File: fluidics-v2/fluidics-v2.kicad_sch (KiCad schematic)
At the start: 25 parts, among them J1 PJ-063AH, J10 87832-1010, J11 87832-1010, J12 87832-1010, J13 0533980671, J14 0533980671, J15 A-DS_15_A_KG-T4S, J2 0705430001, J3 0705430001, J4 0705430001, J5 0705430001, J6 0705430001, J7 1860280, J8 87832-1010, J9 87832-1010, U2 Teensy4.1

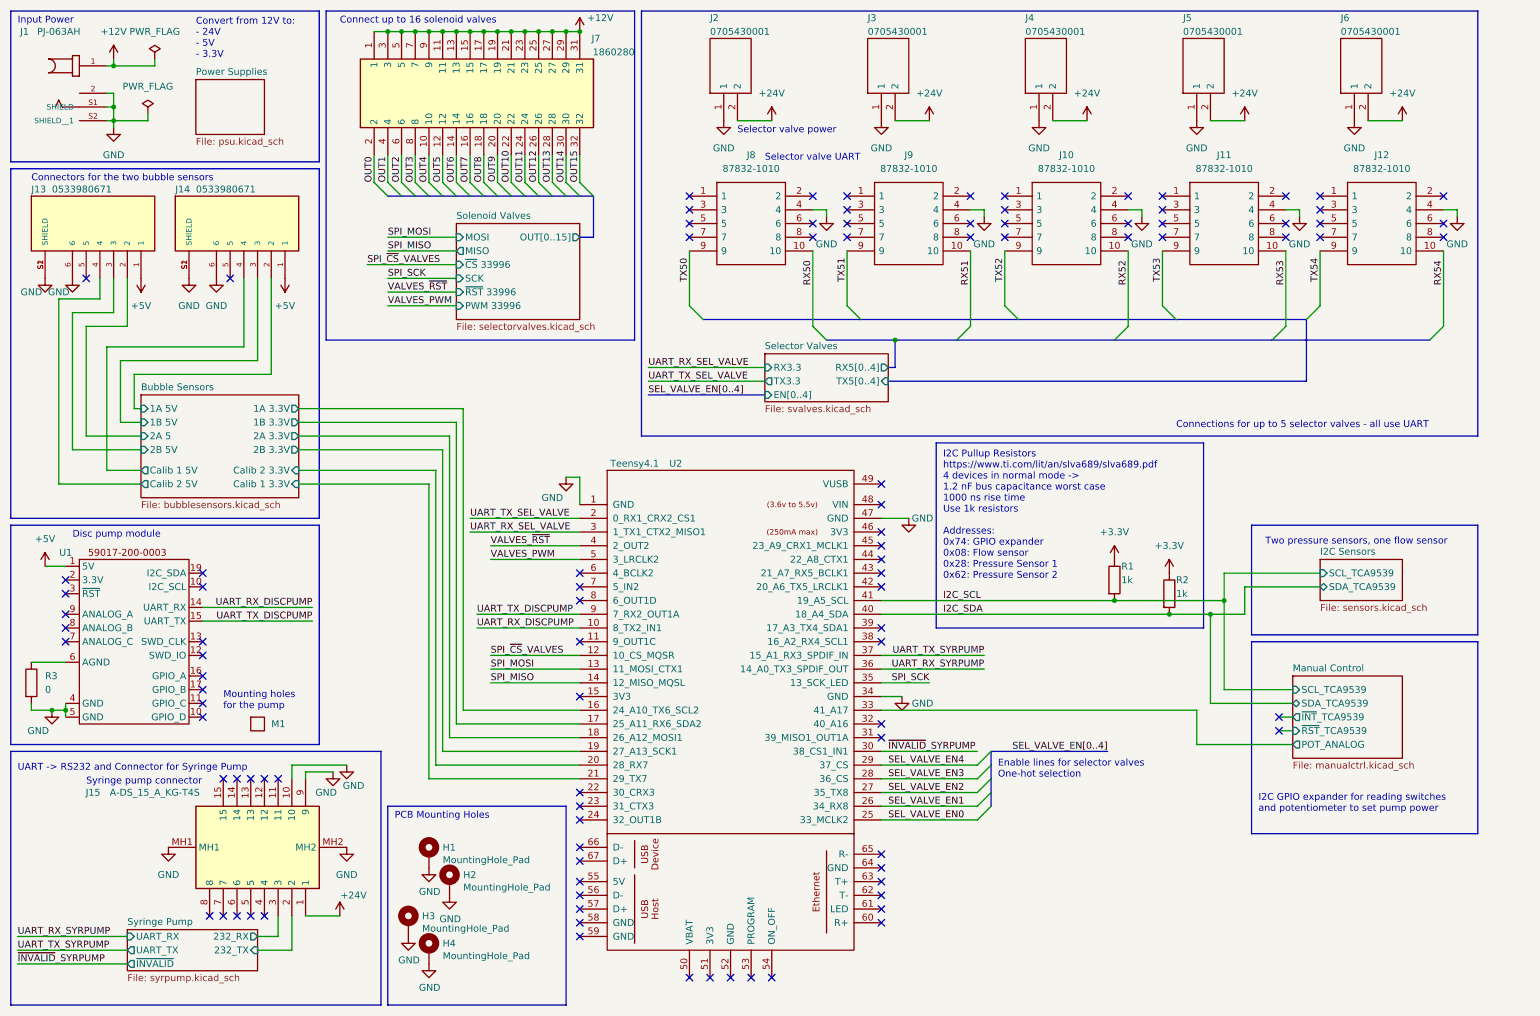
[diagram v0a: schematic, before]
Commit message: new version
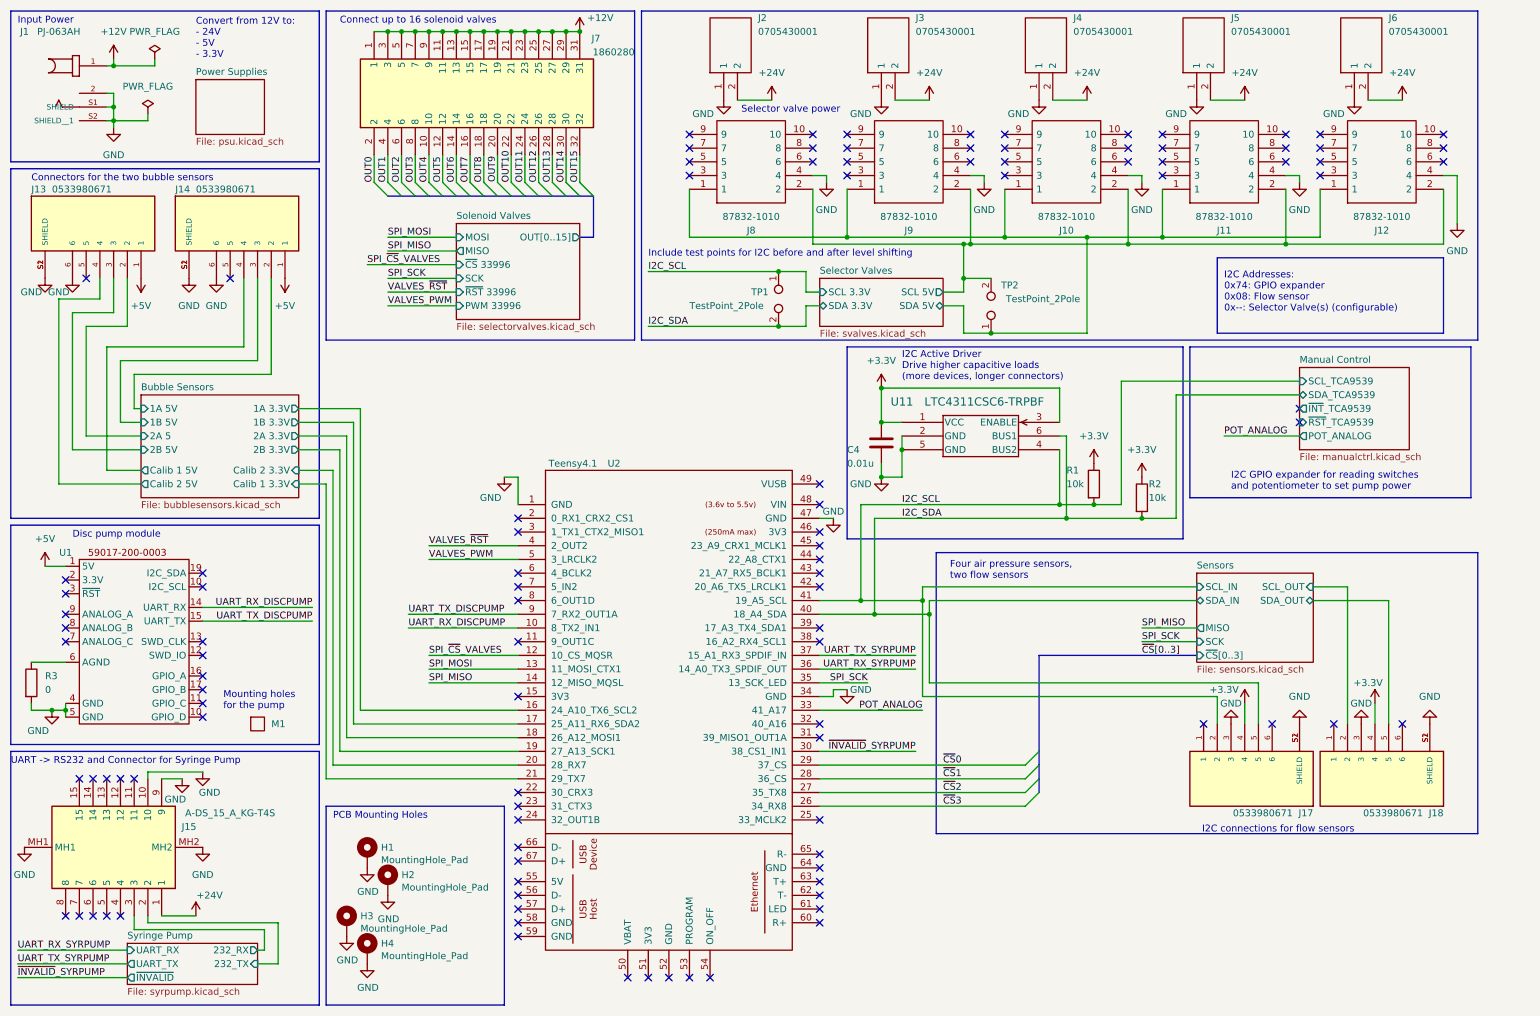
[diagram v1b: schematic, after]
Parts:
- added C4: 0.01u, Capacitor_SMD:C_0603_1608Metric, symbol Device:C
- added J17, J18: 0533980671, molex_connectors:MOLEX_0533980671, symbol 0533980671:0533980671
- added TP1, TP2: TestPoint_2Pole, TestPoint:TestPoint_2Pads_Pitch2.54mm_Drill0.8mm, symbol Connector:TestPoint_2Pole
- added U11: LTC4311CSC6-TRPBF, SOT-6_SC_LIT, symbol LTC4311CSC6#TRPBF:LTC4311CSC6-TRPBF
- R1, R2: value 1k -> 10k
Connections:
- net +3.3V: now also C4.1, J17.4, J18.4, U11.1 (VCC), U11.3 (ENABLE)
- net GND: now also C4.2, J17.3, J17.S1 (SHIELD), J17.S2 (SHIELD), J18.3, J18.S1 (SHIELD), J18.S2 (SHIELD), U11.2 (GND), U11.5 (GND)
- net I2C_SCL: now also J17.2, TP1.1, U11.4 (BUS2)
- net I2C_SDA: now also J17.5, TP1.2, U11.6 (BUS1)
- net Selector Valves/SDA 5V: now reaches J12.1
- net Selector Valves/SDA 5V: now also J10.1, J11.1, J8.1, J9.1, TP2.1
- net Selector Valves/SCL 5V: now reaches J12.2
- net Selector Valves/SCL 5V: now also J10.2, J11.2, J8.2, J9.2, TP2.2
- net Manual Control/POT_ANALOG renamed POT_ANALOG
- net RX50: no longer names the net of J8.10
- net RX51: no longer names the net of J9.10
- net RX52: no longer names the net of J10.10
- net RX53: no longer names the net of J11.10
- net RX54: no longer names the net of J12.10
- net SEL_VALVE_EN0: no longer names the net of U2.25 (33_MCLK2)
- net SEL_VALVE_EN1 renamed ~{CS}3
- net SEL_VALVE_EN2 renamed ~{CS}2
- net SEL_VALVE_EN3 renamed ~{CS}1
- net SEL_VALVE_EN4 renamed ~{CS}0
- net TX50: no longer names the net of J8.9
- net TX51: no longer names the net of J9.9
- net TX52: no longer names the net of J10.9
- net TX53: no longer names the net of J11.9
- net TX54: no longer names the net of J12.9
- net UART_RX_SEL_VALVE: no longer names the net of U2.3 (1_TX1_CTX2_MISO1)
- net UART_TX_SEL_VALVE: no longer names the net of U2.2 (0_RX1_CRX2_CS1)
- new net Sensors/SCL_OUT: J18.2
- new net Sensors/SDA_OUT: J18.5
- no-connect marks 99 -> 106
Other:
- sheet I2C Sensors renamed Sensors
- sheet Selector Valves ports: added SCL 3.3V, SCL 5V, SDA 3.3V, SDA 5V; removed EN[0..4], RX3.3, RX5[0..4], TX3.3, TX5[0..4]
- sheet Sensors ports: added MISO, SCK, SCL_IN, SCL_OUT, SDA_IN, SDA_OUT, ~{CS}[0..3]; removed SCL_TCA9539, SDA_TCA9539
- note added: "Four air pressure sensors, two flow sensors"
- note added: "I2C Active Driver Drive higher capacitive loads (more devices, longer connectors)"
- note added: "I2C Addresses: 0x74: GPIO expander 0x08: Flow sensor 0x--: Selector Valve(s) (configurable)"
- note added: "I2C connections for flow sensors"
- note added: "Include test points for I2C before and after level shifting"
- note removed: "Connections for up to 5 selector valves - all use UART"
- note removed: "Enable lines for selector valves One-hot selection"
- note removed: "I2C Pullup Resistors https://www.ti.com/lit/an/slva689/slva689.pdf 4 devices in normal mode -> 1.2 nF bus capacitance worst case 1000 ns rise time Use 1k resistors Addresses: 0x74: GPIO expander 0x08: Flow sensor 0x28: Pressure Sensor 1 0x62: Pressure Sensor 2"
- note removed: "Selector valve UART"
- note removed: "Syringe pump connector"
- note removed: "Two pressure sensors, one flow sensor"
- moved on the sheet: H1, H2, H3, H4, J10, J11, J12, J15, J2, J3, J4, J5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
